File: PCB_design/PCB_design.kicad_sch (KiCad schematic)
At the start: 2 parts, among them U1 L298N

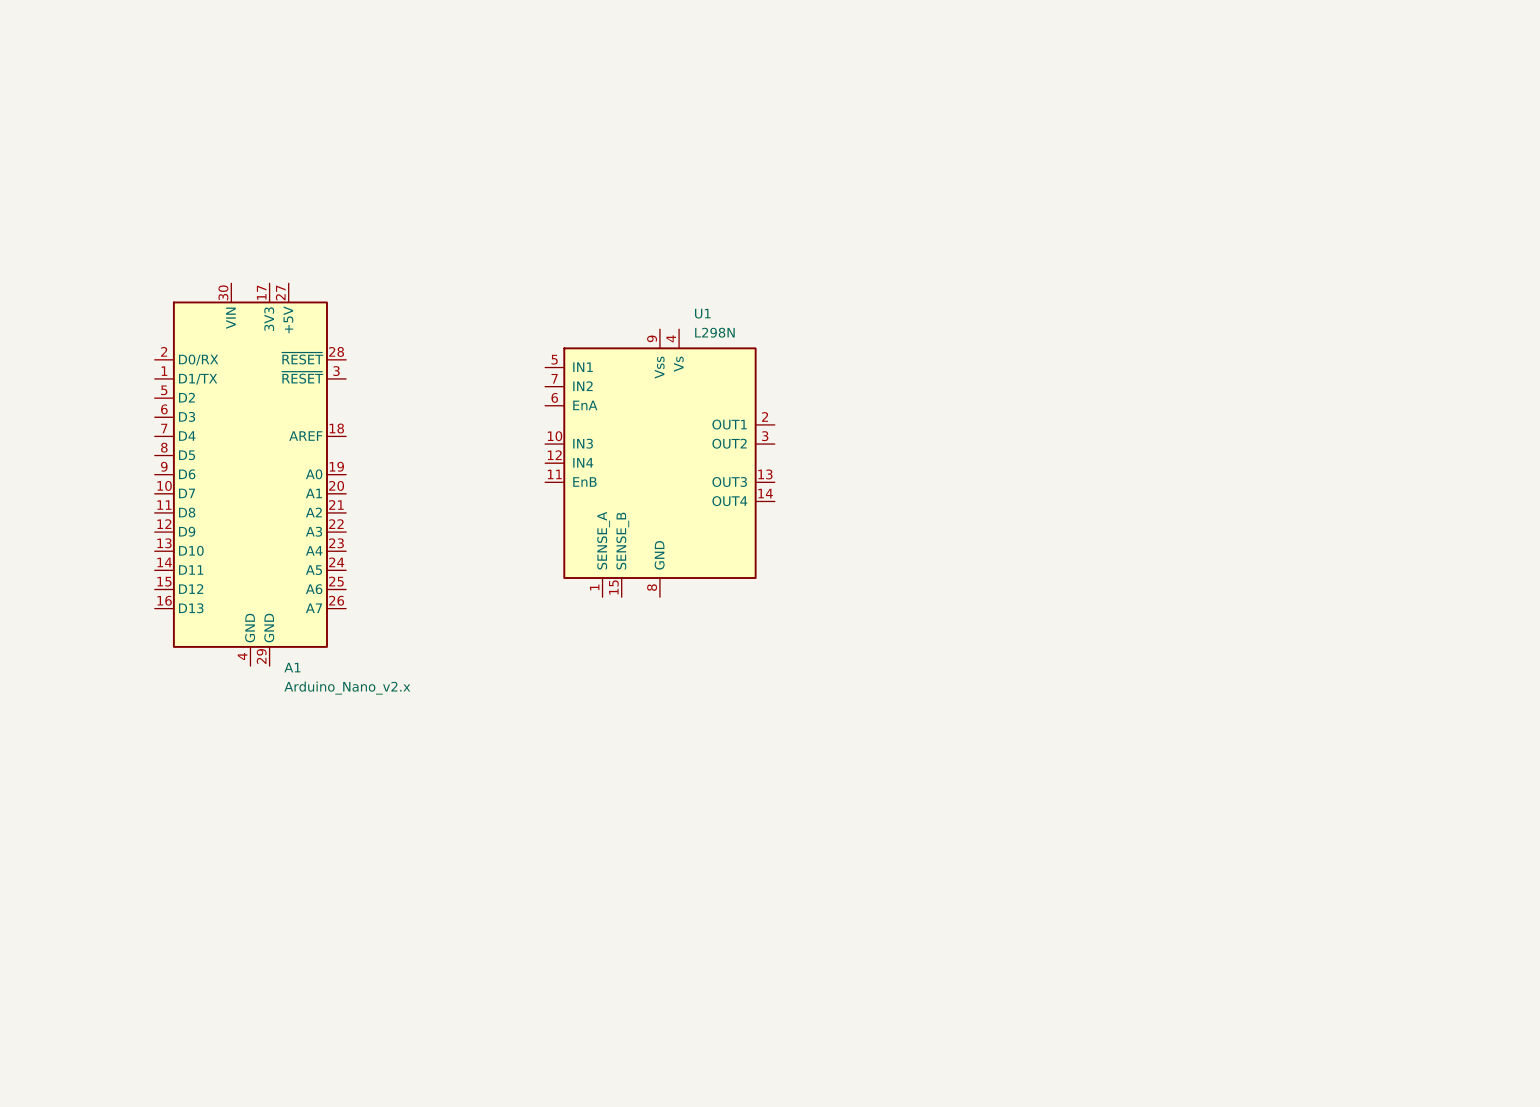
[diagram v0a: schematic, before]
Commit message: Updated PCB Design
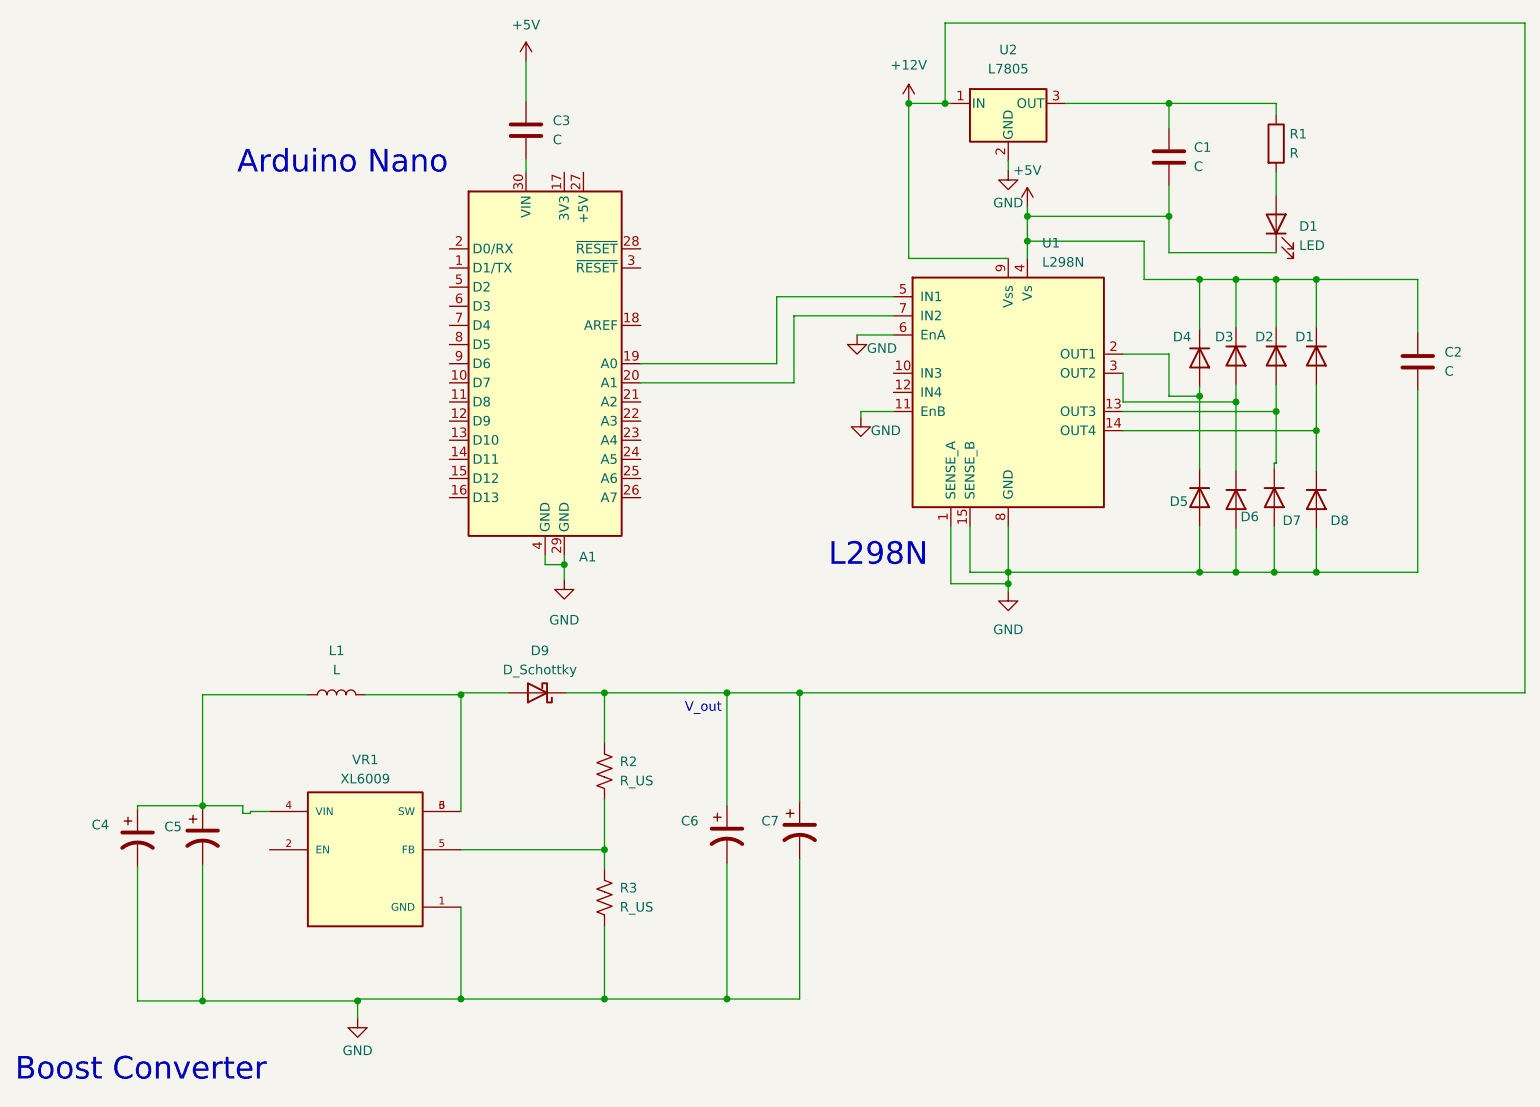
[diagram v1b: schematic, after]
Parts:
- added C1, C2, C3: C, symbol Device:C
- added C4, C5, C6, C7: C_Polarized_US, symbol Device:C_Polarized_US
- added D1: LED, symbol Device:LED
- added D1, D2, D3, D4, D5, D6, D7, D8: 1N5400, Diode_THT:D_DO-201AD_P15.24mm_Horizontal, symbol Diode:1N5400
- added D9: D_Schottky, symbol Device:D_Schottky
- added L1: L, symbol Device:L
- added R1: R, symbol Device:R
- added R2, R3: R_US, symbol Device:R_US
- added U2: L7805, symbol Regulator_Linear:L7805
- added VR1: XL6009, XL6009:DPAK170P1435X465-6N, symbol XL6009:XL6009
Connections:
- net GND: now reaches U1.1 (SENSE_A)
- net GND: now also A1.29 (GND), A1.4 (GND), U1.11 (EnB), U1.15 (SENSE_B), U1.6 (EnA), U1.8 (GND), C2.2, C4.2, C5.2, C6.2, C7.2, D5.2 (A), D6.2 (A), D7.2 (A), D8.2 (A), R3.2, U2.2 (GND), VR1.1 (GND)
- net at U1.13 (OUT3): now also D2.2 (A), D7.1 (K)
- net at U1.14 (OUT4): now also D1.2 (A), D8.1 (K)
- net at U1.2 (OUT1): now also D4.2 (A), D5.1 (K)
- net at U1.3 (OUT2): now also D3.2 (A), D6.1 (K)
- net +5V: now reaches U1.4 (Vs)
- net +5V: now also C1.2, C2.1, C3.1, D1.1 (K), D1.1 (K), D2.1 (K), D3.1 (K), D4.1 (K)
- net at U1.5 (IN1): now also A1.19 (A0)
- net at U1.7 (IN2): now also A1.20 (A1)
- net +12V: now reaches U1.9 (Vss)
- net +12V: now also C6.1, C7.1, D9.1 (K), R2.1, U2.1 (IN)
- net at A1.30 (VIN): now also C3.2
- new net: C4.1, C5.1, L1.1, VR1.4 (VIN)
- new net: C1.1, R1.1, U2.3 (OUT)
- new net: D1.2 (A), R1.2
- new net: D9.2 (A), L1.2, VR1.3 (SW), VR1.6 (SW)
- new net: R2.2, R3.1, VR1.5 (FB)
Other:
- note added: "Arduino Nano"
- note added: "Boost Converter"
- note added: "L298N"
- note added: "V_out"
- moved on the sheet: A1, U1
